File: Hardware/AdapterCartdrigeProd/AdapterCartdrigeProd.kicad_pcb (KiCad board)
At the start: 2 copper layers, 41.5 x 83.9 mm, 5 parts, among them J1 ROM, U1 28C256

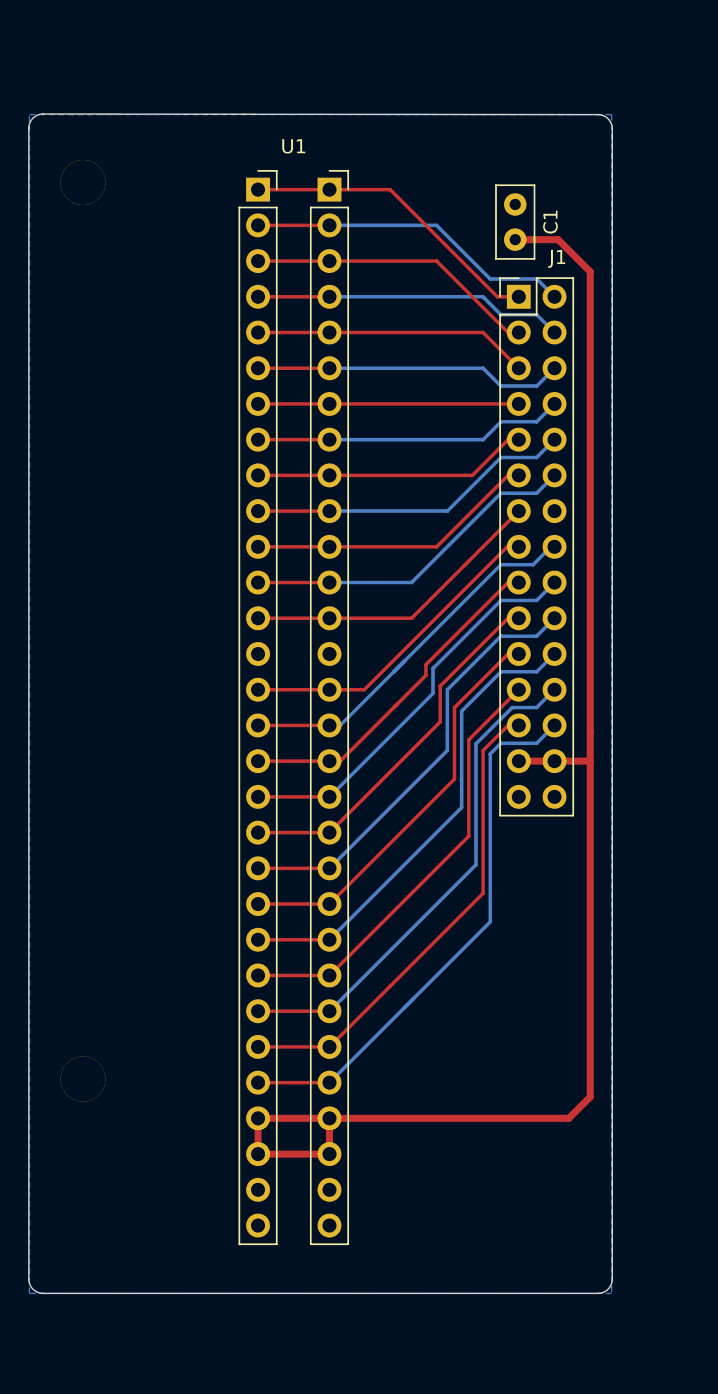
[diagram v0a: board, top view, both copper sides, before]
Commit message: Fix
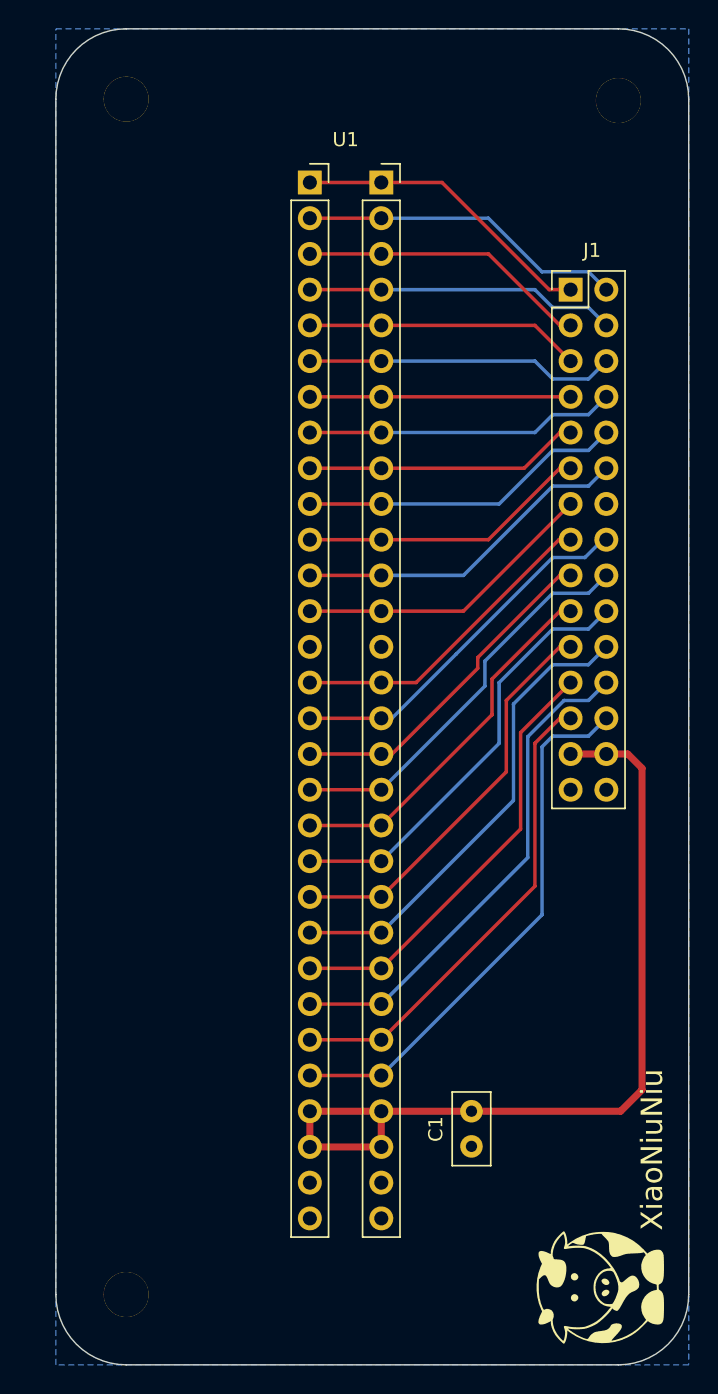
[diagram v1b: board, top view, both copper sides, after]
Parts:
- added H3: MountingHole_Pad, MountingHole:MountingHole_3.2mm_M3, F.Cu at (129.0, 37.1)
- added XiaoNiuNiu: LOGO, Logos:VerySmallCow, F.Cu at (127.7, 121.5)
- moved C1 62.1 mm to (118.6, 109.0), turned to -90 degrees
- moved H2 15.6 mm to (94.0, 122.0)
- moved H1 6.67 mm to (94.0, 37.0)
- moved J1 3.72 mm to (125.6, 50.5)
- moved U1 3.72 mm to (109.6, 79.8)
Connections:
- H1 pad : (no net) -> GND
- H2 pad : (no net) -> GND
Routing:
- net +5V: track 104.7 -> 62.8 mm
- net /D4: track 27.4 -> 26.1 mm
- net /A13: track 39.5 -> 38.6 mm
- net /A14: track 22.2 -> 21.7 mm
- net /D3: track 23.3 -> 22.8 mm
- net GND: track 0.51 -> 0.00 mm
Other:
- board size 41.5 x 83.9 mm -> 45 x 95 mm
